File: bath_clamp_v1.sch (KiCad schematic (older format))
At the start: 18 parts, among them U10 LP2951-3.3_SOIC, U7 LM337L_SO8, U9 MCP1804x-3302xOT

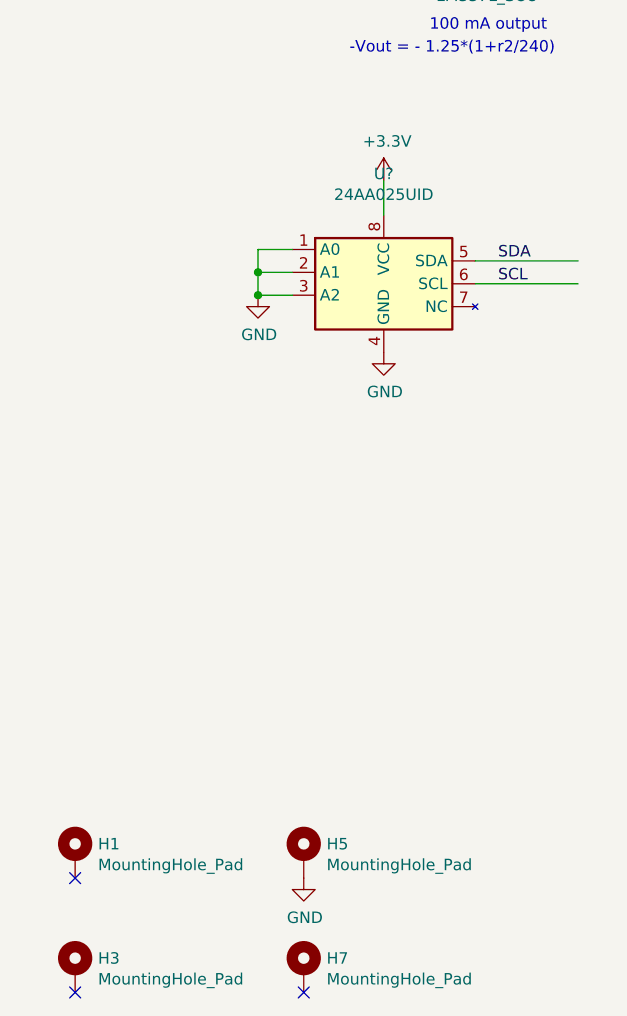
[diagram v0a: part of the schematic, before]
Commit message: updates to pcb layout
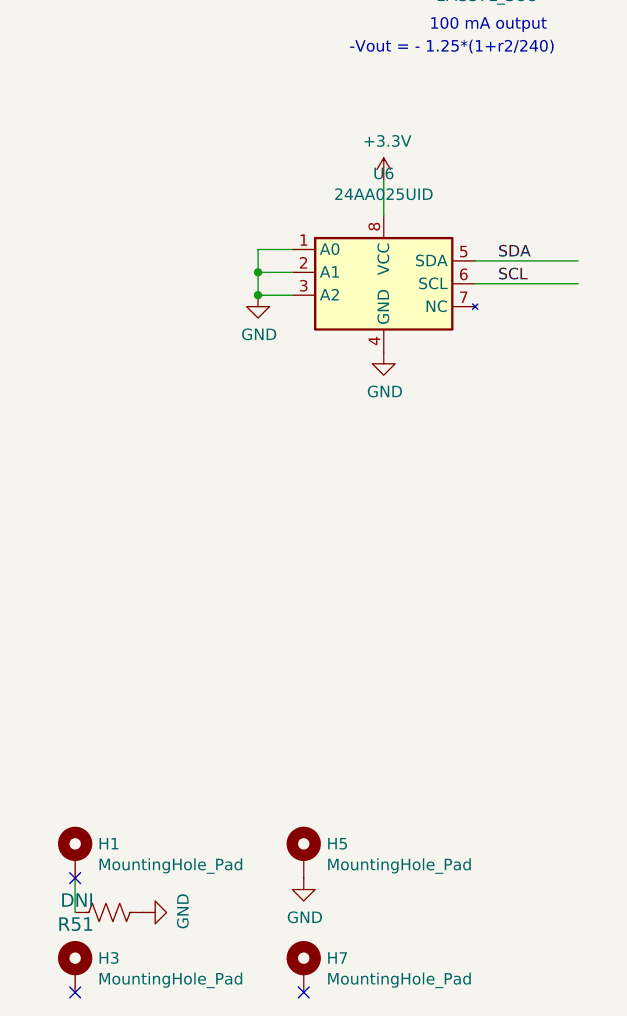
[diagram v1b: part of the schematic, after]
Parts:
- added R51: DNI, Resistor_SMD:R_0603_1608Metric, symbol Device:R_US
- H1, H3, H5, H7: footprint (none) -> MountingHole:MountingHole_3.2mm_M3_DIN965_Pad
- gave numbers to parts that had none: 1
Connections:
- wire segments 61 -> 62
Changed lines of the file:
@@
 F 0 "H1" H 1000 6899 50  0000 L CNN
 F 1 "MountingHole_Pad" H 1000 6808 50  0000 L CNN
-F 2 "" H 900 6850 50  0001 C CNN
+F 2 "MountingHole:MountingHole_3.2mm_M3_DIN965_Pad" H 900 6850 50  0001 C CNN
 F 3 "~" H 900 6850 50  0001 C CNN
 	1    900  6850
@@
 F 0 "H3" H 1000 7399 50  0000 L CNN
 F 1 "MountingHole_Pad" H 1000 7308 50  0000 L CNN
-F 2 "" H 900 7350 50  0001 C CNN
+F 2 "MountingHole:MountingHole_3.2mm_M3_DIN965_Pad" H 900 7350 50  0001 C CNN
 F 3 "~" H 900 7350 50  0001 C CNN
 	1    900  7350
@@
 F 0 "H7" H 2000 7399 50  0000 L CNN
 F 1 "MountingHole_Pad" H 2000 7308 50  0000 L CNN
-F 2 "" H 1900 7350 50  0001 C CNN
+F 2 "MountingHole:MountingHole_3.2mm_M3_DIN965_Pad" H 1900 7350 50  0001 C CNN
 F 3 "~" H 1900 7350 50  0001 C CNN
 	1    1900 7350
@@
 F 0 "H5" H 2000 6899 50  0000 L CNN
 F 1 "MountingHole_Pad" H 2000 6808 50  0000 L CNN
-F 2 "" H 1900 6850 50  0001 C CNN
+F 2 "MountingHole:MountingHole_3.2mm_M3_DIN965_Pad" H 1900 6850 50  0001 C CNN
 F 3 "~" H 1900 6850 50  0001 C CNN
 	1    1900 6850
@@
 SDA
 $Comp
-L covg-kicad:24AA025UID U?
+L covg-kicad:24AA025UID U6
 U 1 1 627267F8
 P 2250 4350
-F 0 "U?" H 2250 4831 50  0000 C CNN
+F 0 "U6" H 2250 4831 50  0000 C CNN
 F 1 "24AA025UID" H 2250 4740 50  0000 C CNN
 F 2 "Package_SO:SOIC-8_3.9x4.9mm_P1.27mm" H 2250 4350 50  0001 C CNN
@@
 	1    0    0    -1
 $EndComp
+$Comp
+L Device:R_US R?
+U 1 1 6277A90A
+P 1050 7100
+AR Path="/6032F251/6277A90A" Ref="R?"  Part="1"
+AR Path="/6277A90A" Ref="R51"  Part="1"
+F 0 "R51" V 997 7168 59  0000 L CNN
+F 1 "DNI" V 1102 7168 59  0000 L CNN
+F 2 "Resistor_SMD:R_0603_1608Metric" H 1050 7100 50  0001 C CNN
+F 3 "" H 1050 7100 50  0001 C CNN
+F 4 "RC0603FR-07240RL" H 997 7268 50  0001 C CNN "Manf#"
+F 5 "1%" H 1050 7100 50  0001 C CNN "Tolerance"
+	1    1050 7100
+	0    -1   -1   0
+$EndComp
+$Comp
+L power:GND #PWR0136
+U 1 1 6277B1AB
+P 1200 7100
+F 0 "#PWR0136" H 1200 6850 50  0001 C CNN
+F 1 "GND" H 1205 6927 50  0000 C CNN
+F 2 "" H 1200 7100 50  0001 C CNN
+F 3 "" H 1200 7100 50  0001 C CNN
+	1    1200 7100
+	0    -1   -1   0
+$EndComp
+Wire Wire Line
+	900  7100 900  6950
 $EndSCHEMATC

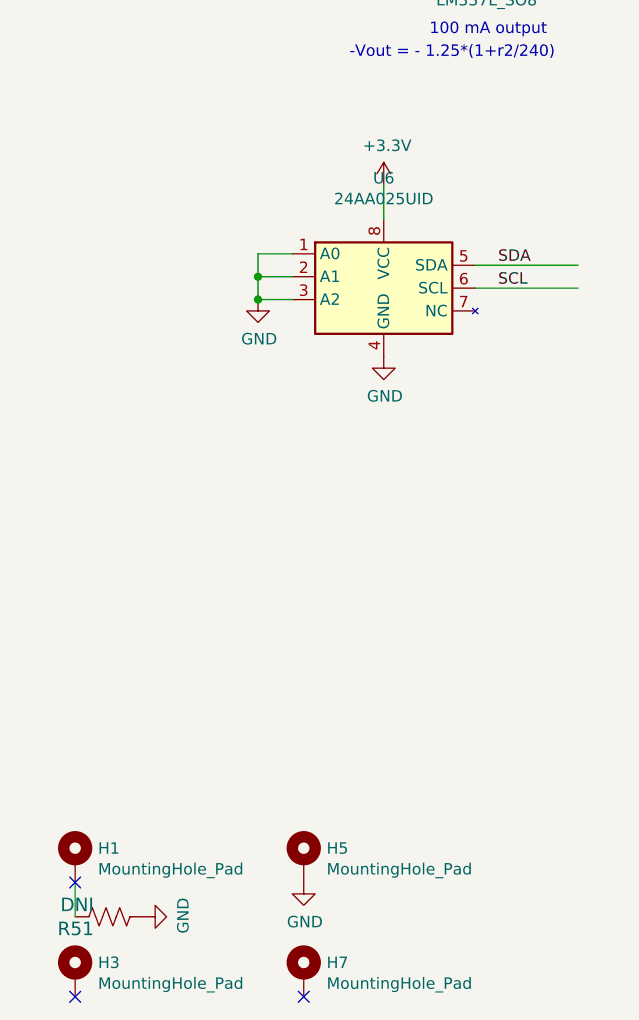
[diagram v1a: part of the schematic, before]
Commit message: made sheet for Howland
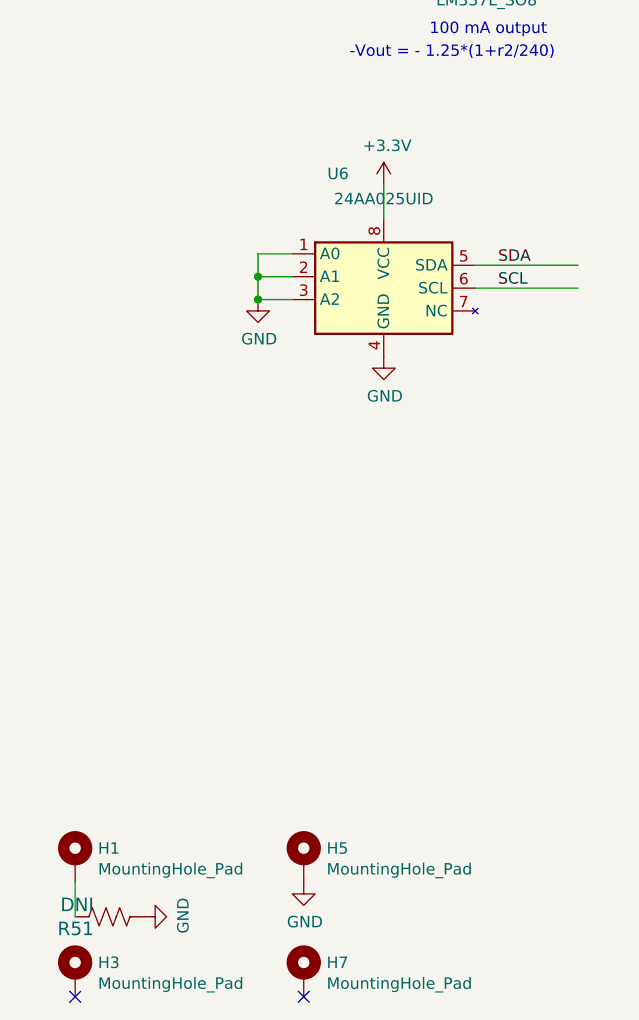
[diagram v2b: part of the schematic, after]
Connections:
- no-connect marks 5 -> 4
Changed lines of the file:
@@
 $Descr A4 11693 8268
 encoding utf-8
-Sheet 1 6
+Sheet 1 7
 Title "Bath/Guard Clamp"
 Date "2021-04-06"
@@
 NoConn ~ 8600 2750
 NoConn ~ 8600 2950
-NoConn ~ 900  6950
 NoConn ~ 900  7450
 NoConn ~ 1900 7450
@@
 U 1 1 627267F8
 P 2250 4350
-F 0 "U6" H 2250 4831 50  0000 C CNN
+F 0 "U6" H 2050 4850 50  0000 C CNN
 F 1 "24AA025UID" H 2250 4740 50  0000 C CNN
 F 2 "Package_SO:SOIC-8_3.9x4.9mm_P1.27mm" H 2250 4350 50  0001 C CNN
@@
 $EndComp
 Wire Wire Line
-	900  7100 900  6950
+	900  6950 900  7100
 $EndSCHEMATC
